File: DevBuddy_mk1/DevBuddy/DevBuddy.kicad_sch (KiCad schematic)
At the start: 7 parts, among them U1 RP2354B

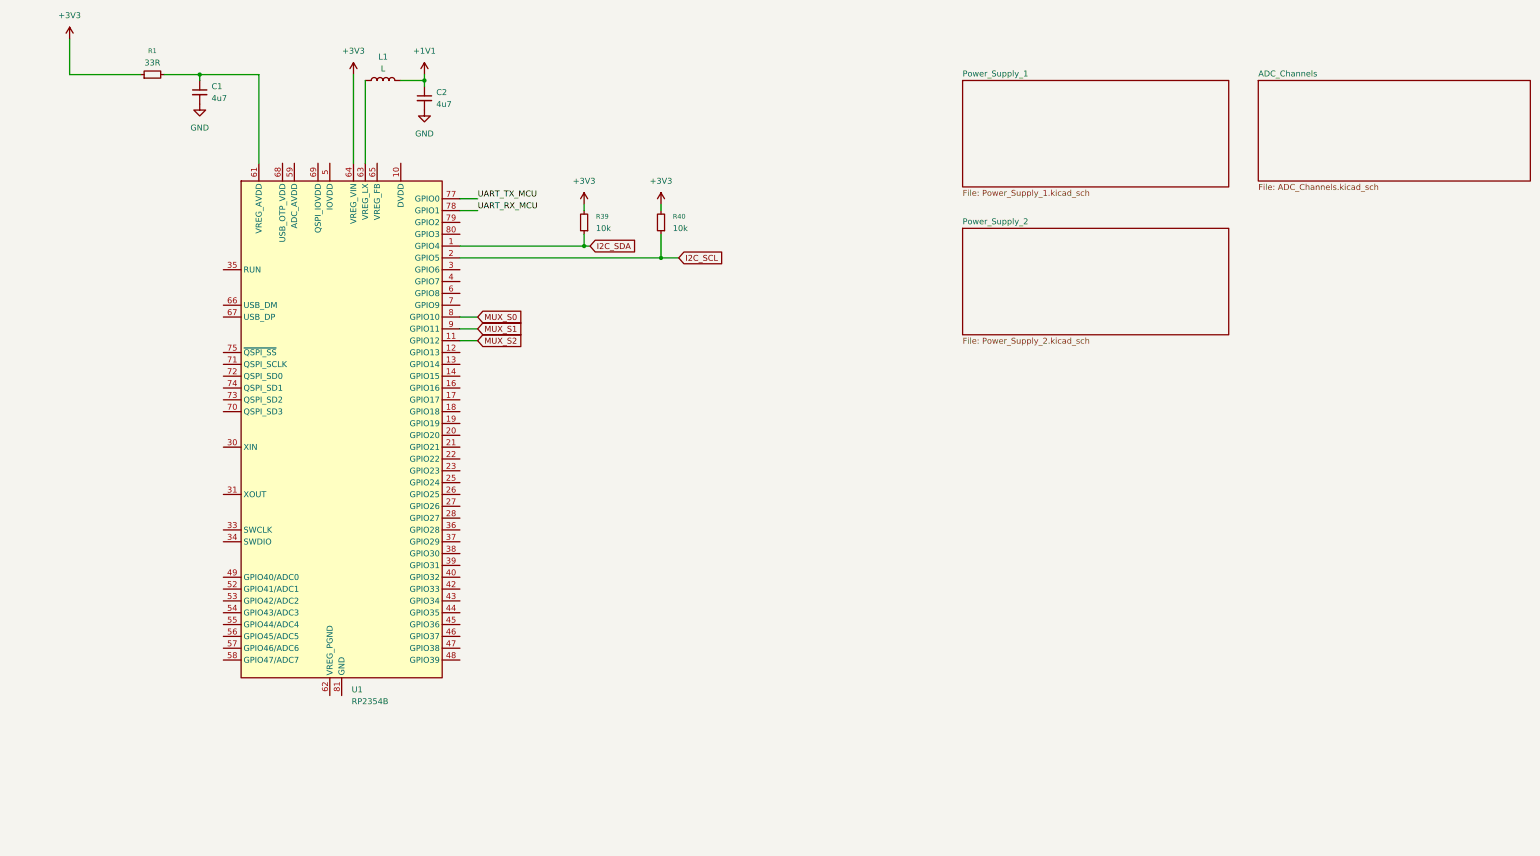
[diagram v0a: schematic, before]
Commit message: Heavy additions to schematic
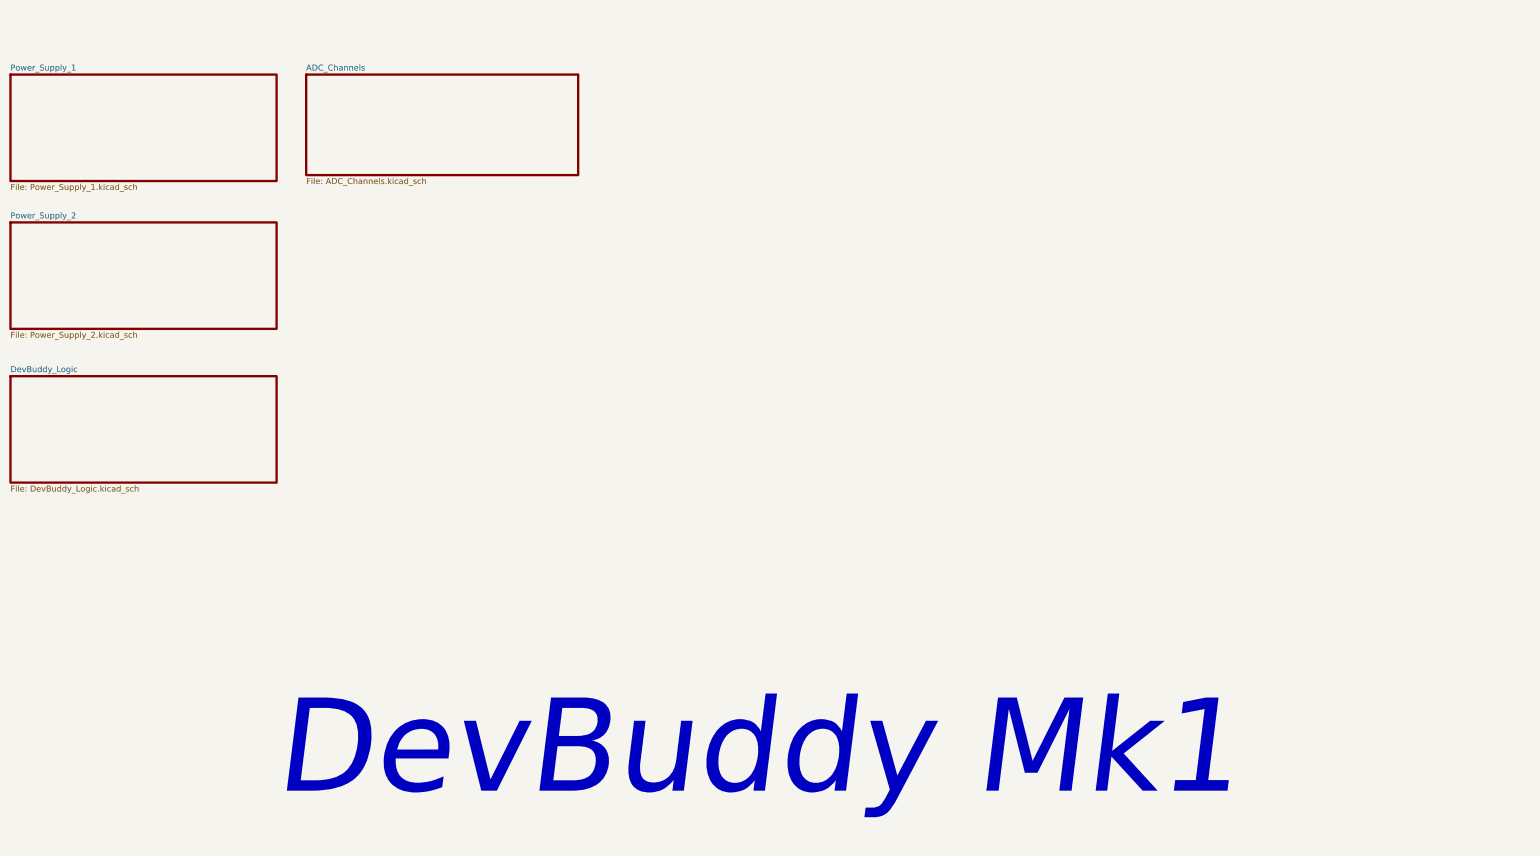
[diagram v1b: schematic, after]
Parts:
- removed C1, C2: 4u7, Capacitor_SMD:C_0402_1005Metric, symbol Device:C_Small
- removed L1: L, Inductor_SMD:L_Coilcraft_0805HQ_2012Metric, symbol Device:L
- removed R1: 33R, Resistor_SMD:R_0402_1005Metric, symbol Device:R_Small
- removed R39, R40: 10k, Resistor_SMD:R_0402_1005Metric, symbol Device:R_Small
- removed U1: RP2354B, Package_DFN_QFN:QFN-80-1EP_10x10mm_P0.4mm_EP3.4x3.4mm, symbol MCU_RaspberryPi:RP2354B
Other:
- added sheet DevBuddy_Logic (DevBuddy_Logic.kicad_sch)
- note added: "DevBuddy Mk1"
